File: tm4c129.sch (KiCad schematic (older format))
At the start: 44 parts, among them SW401 RST_SW, U401 TM4C1294NCPDTGOOD, Y401 Crystal_GND24, Y402 Crystal

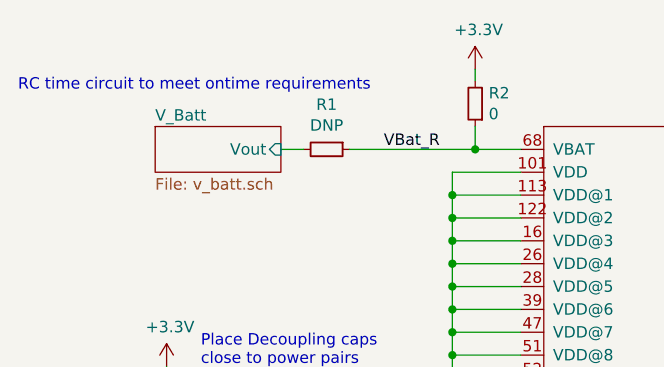
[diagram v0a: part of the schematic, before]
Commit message: layout and schematic cleanup.
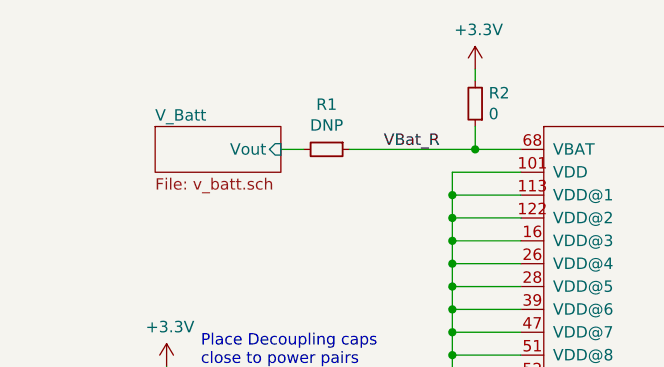
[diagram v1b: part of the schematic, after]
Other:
- note removed: "RC time circuit to meet ontime requirements"
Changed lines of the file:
@@
 F2 "Vout" I R 1700 1050 50
 $EndSheet
-Text Notes 550  800  0    50   ~ 0
-RC time circuit to meet ontime requirements
 Wire Wire Line
 	1700 1050 1800 1050
